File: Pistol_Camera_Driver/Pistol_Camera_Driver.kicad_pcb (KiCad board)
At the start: 2 copper layers, 95.8 x 38.7 mm, 58 parts, among them J1 Strobe, J10 Bluetooth, J11 reserve, J12 reserve, J2 Objective, J3 Screw_Terminal_01x02, J4 Screw_Terminal_01x02, J5 SONAR, J6 Joystick, J7 Screw_Terminal_01x02, J8 test, J9 Screw_Terminal_01x02, U1 LM7805_TO220, U10 RS0101YH6, U11 LDD-700L, U2 LM317_TO-263, U3 Raspberri_Pi_Pico, U4 DRV8834PWP, U5 DRV8834PWP, U6 RS0101YH6, U7 LDD-700L, U8 RS0101YH6, U9 LDD-700L

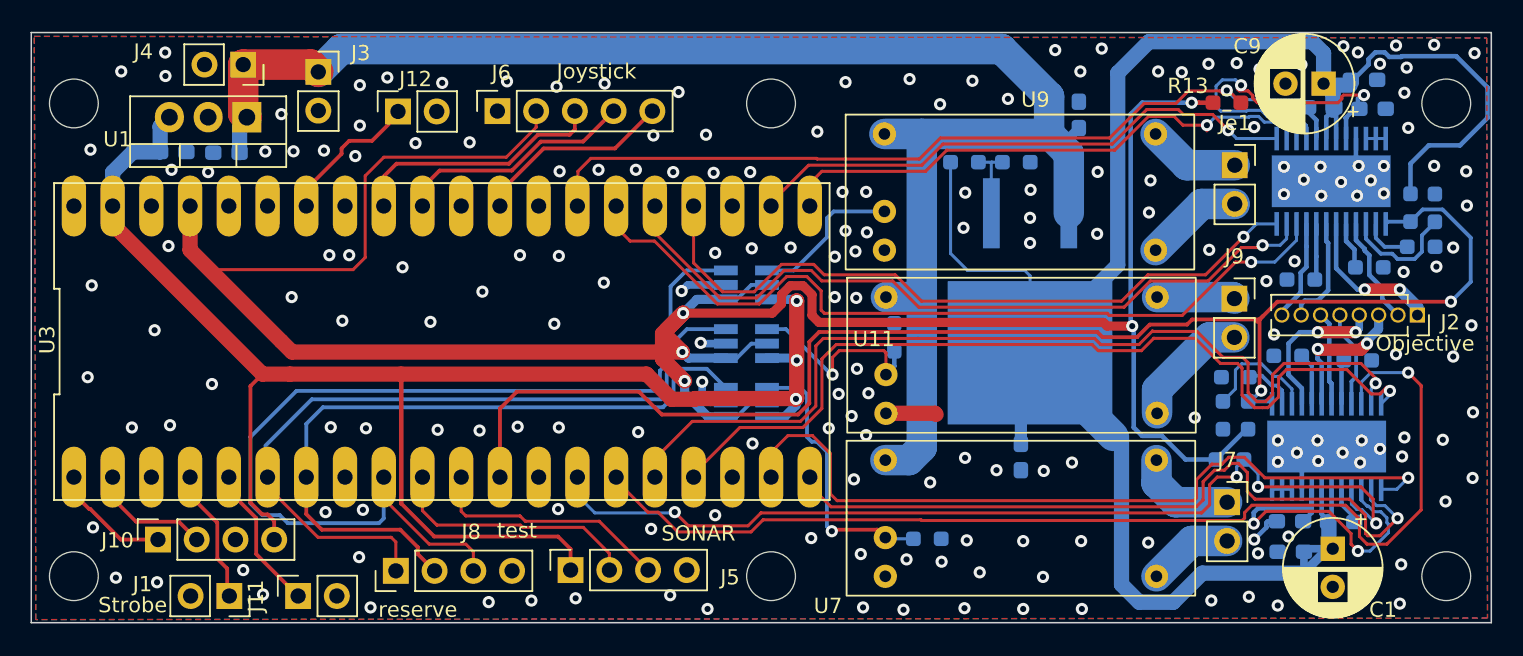
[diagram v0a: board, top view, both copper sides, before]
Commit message: Auto stash before merge of "main" and "origin/main"
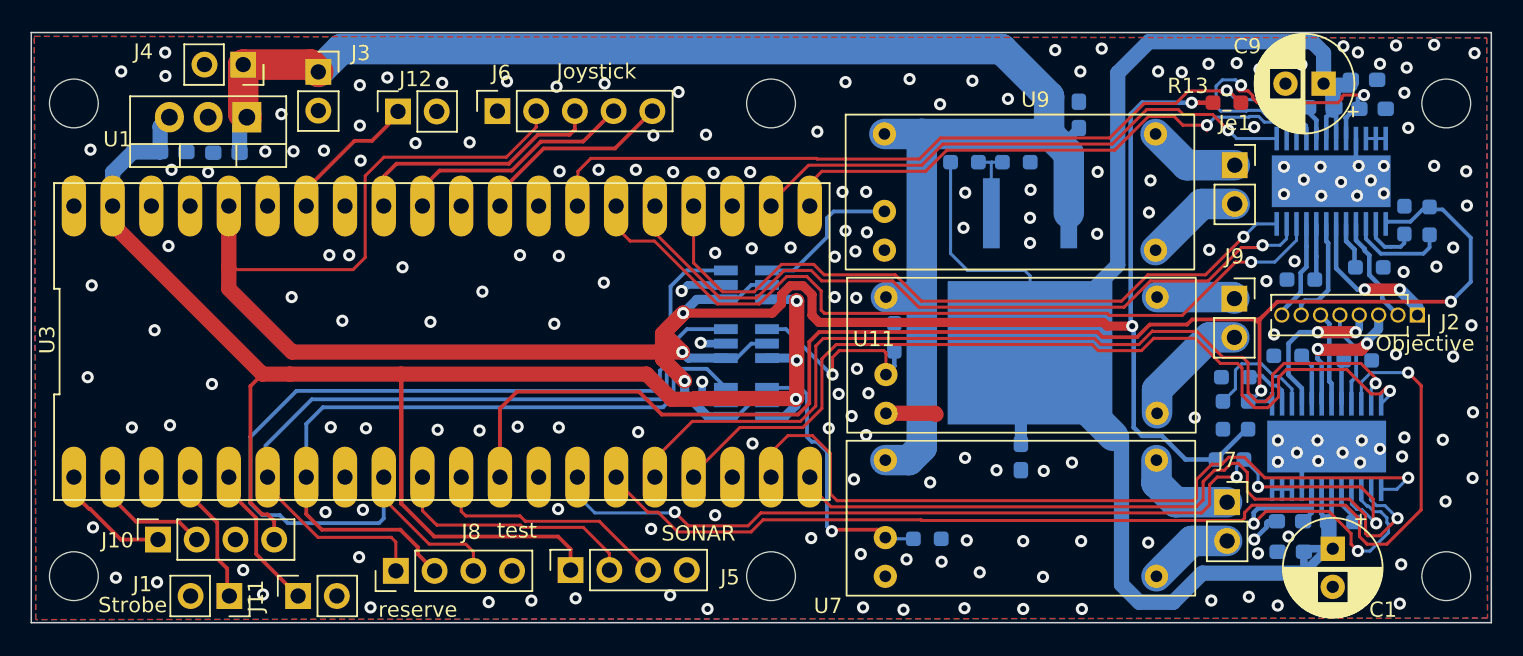
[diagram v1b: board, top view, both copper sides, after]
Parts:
- removed the R9 at (167.1, 35.8)
- R13: value R -> 10 k
- moved R9 2.07 mm to (166.7, 36.6), turned to -90 degrees
- moved R10 0.92 mm to (168.3, 36.7)
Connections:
- U3 pad 36: unconnected-(U3-Pad36) -> +3V3
- U3 pad 37: +3V3 -> unconnected-(U3-Pad37)
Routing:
- net +3.3VP: track 138.3 -> 117.0 mm
- net +3V3: track 169.0 -> 161.8 mm
- net Net-(R10-Pad2): track 7.71 -> 6.56 mm
- net Net-(R9-Pad2): track 3.23 -> 3.73 mm
